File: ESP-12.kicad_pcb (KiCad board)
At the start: 2 copper layers, 30 x 34 mm, 16 parts, among them IC1 REG, P1 GPIO_1, P2 GPIO_2, P3 UART, P4 SPI, P5 P_IN, SW1 RESET, SW2 FLASH, U1 ESP-12E

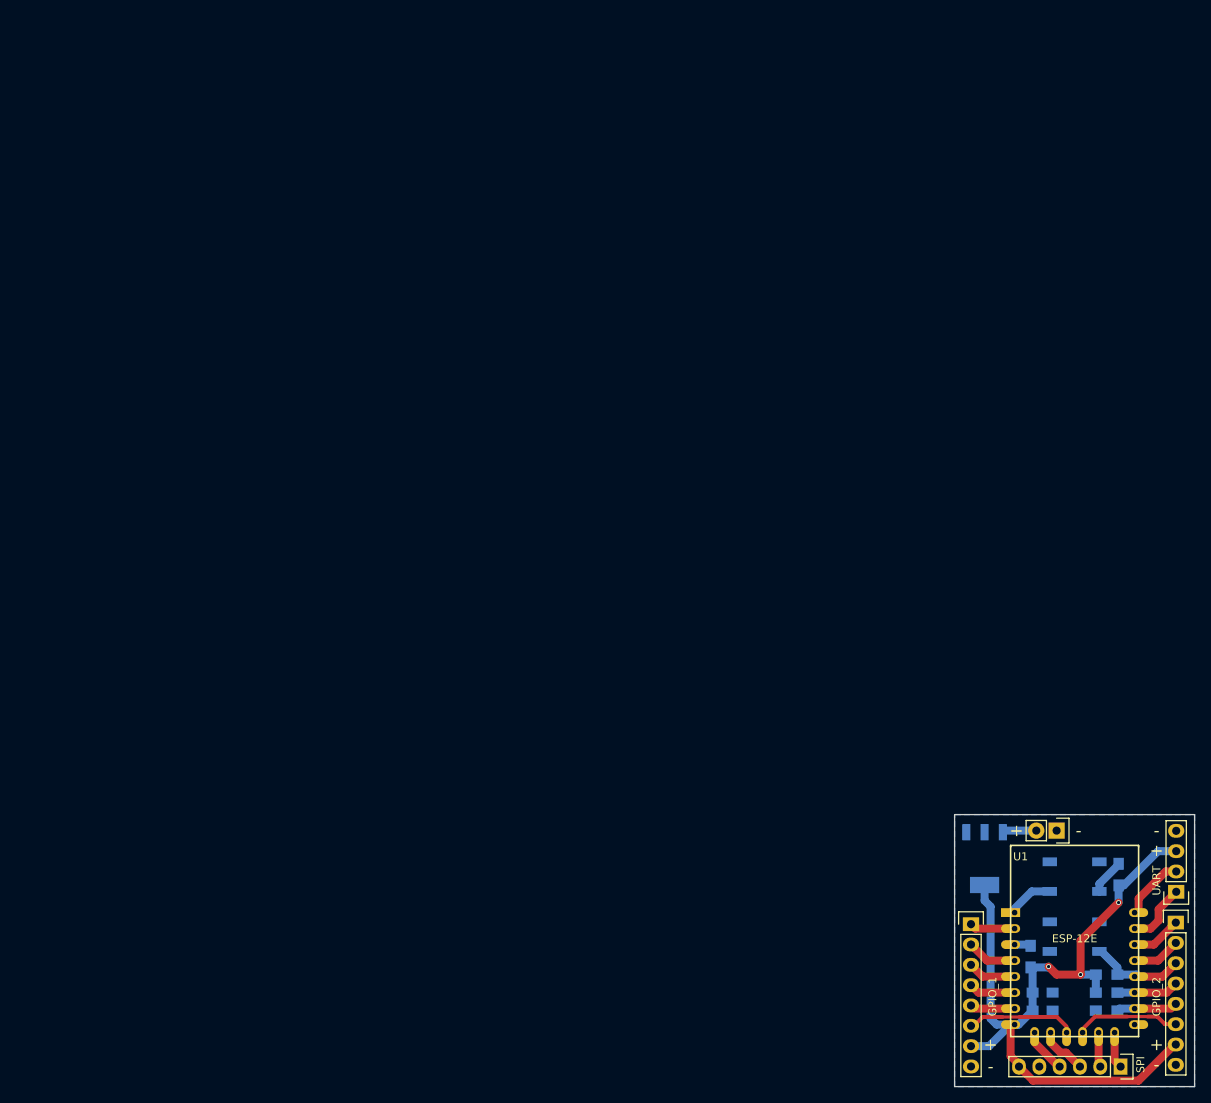
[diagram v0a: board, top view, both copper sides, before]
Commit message: Initial commit
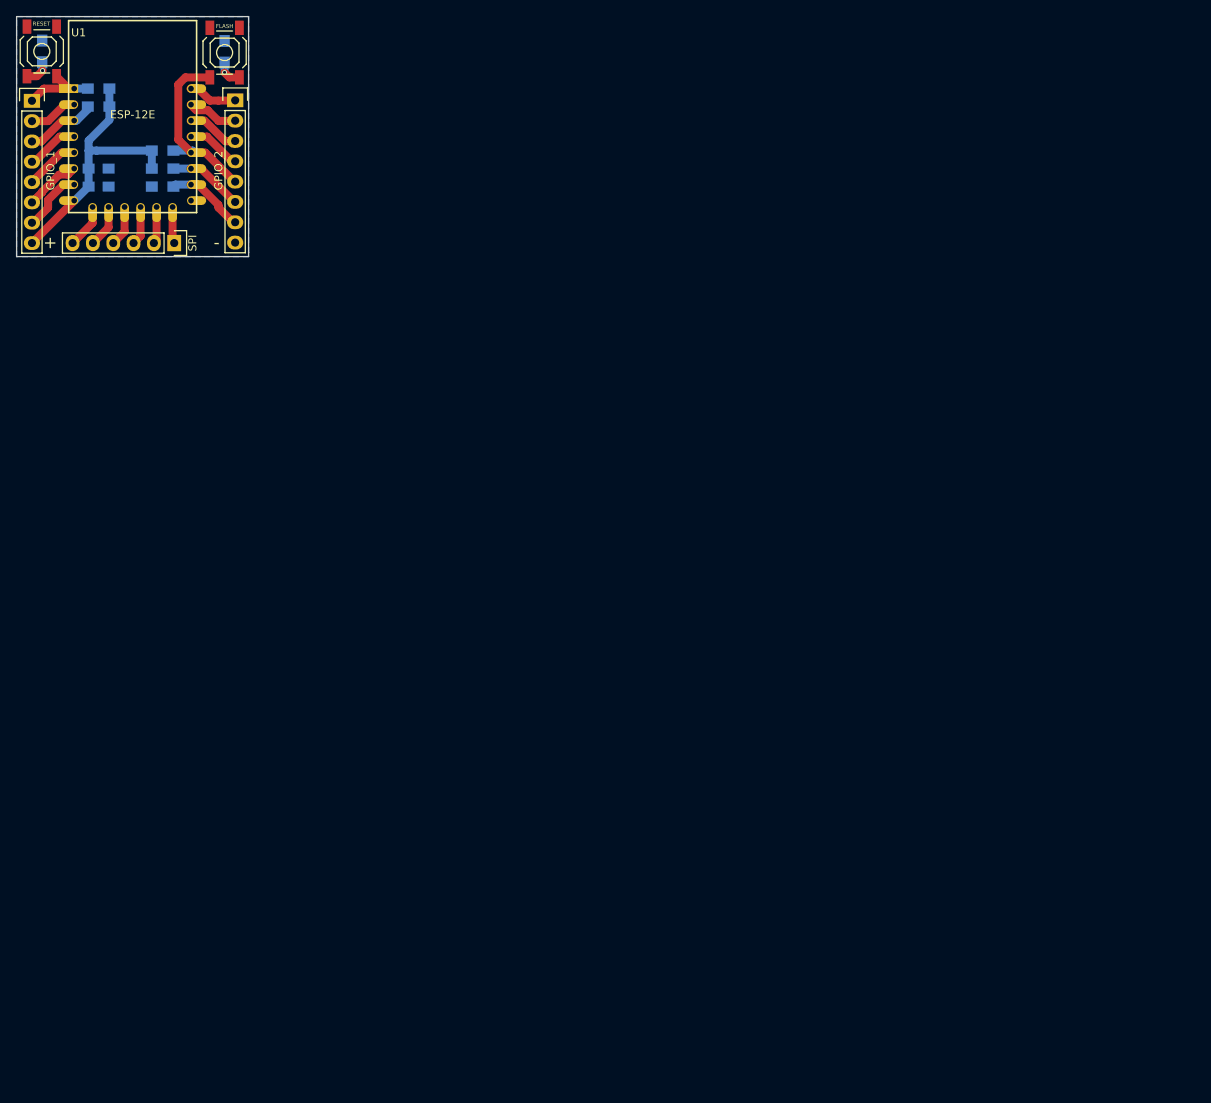
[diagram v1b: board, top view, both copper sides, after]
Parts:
- removed IC1: REG, TO_SOT_Packages_SMD:SOT-223
- removed P4: SPI, Pin_Headers:Pin_Header_Straight_1x06
- removed P5: P_IN, Pin_Headers:Pin_Header_Straight_1x02
- added R6: R, Resistors_SMD:R_0805_HandSoldering, B.Cu at (27.7, 24.1)
- added R7: R, Resistors_SMD:R_0805_HandSoldering, B.Cu at (50.5, 24.1)
- P3: value UART -> SPI; footprint Pin_Headers:Pin_Header_Straight_1x04 -> Pin_Headers:Pin_Header_Straight_1x06
- SW1, SW2: moved to F.Cu
- moved SW1 165.2 mm to (27.6, 24.1), turned to 270 degrees
- moved R1 161.0 mm to (34.8, 28.8), turned to 0 degrees
- moved R2 157.7 mm to (34.8, 31.0), turned to 0 degrees
- moved C2 156.6 mm to (34.8, 41.0)
- moved C3 156.6 mm to (34.8, 38.8)
- moved R3 156.6 mm to (42.8, 36.5)
- moved R4 156.6 mm to (42.8, 38.8)
- moved R5 156.6 mm to (42.8, 41.0)
- moved U1 156.4 mm to (31.0, 28.8)
- moved P2 156.2 mm to (51.8, 30.2)
- moved P1 156.1 mm to (26.4, 30.3)
- moved SW2 153.3 mm to (50.5, 24.2), turned to 90 degrees
- moved P3 149.2 mm to (44.2, 48.1), turned to 270 degrees
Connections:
- P1 pad 1: /ADC -> /RST
- P1 pad 2: /GPIO16 -> /ADC
- P1 pad 3: /GPIO14 -> /CH_PD
- P1 pad 4: /GPIO13 -> /GPIO16
- P1 pad 5: /GPIO12 -> /GPIO14
- P1 pad 6: /GPIO9 -> /GPIO12
- P1 pad 7: VCC -> /GPIO13
- P1 pad 8: GND -> VCC
- R1 pad 1: Net-(R1-Pad1) -> /RST
- R2 pad 1: Net-(R2-Pad1) -> /CH_PD
- SW1 pad 1: Net-(R1-Pad1) -> /RST
- SW1 pad 2: GND -> Net-(R6-Pad2)
- SW2 pad 2: GND -> Net-(R7-Pad2)
- U1 pad 1: Net-(R1-Pad1) -> /RST
- U1 pad 3: Net-(R2-Pad1) -> /CH_PD
- U1 pad 6: /GPIO13 -> /GPIO12
- U1 pad 7: /GPIO12 -> /GPIO13
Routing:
- net VCC: track 95.2 -> 34.4 mm, vias 3 -> 0
- net /GPIO0: track 12.1 -> 23.2 mm
- net Net-(R1-Pad1): track 10.5 -> 0.00 mm
- net /GPIO9: track 14.8 -> 4.89 mm
- net /RST: track 0.00 -> 9.59 mm
- net /GPIO10: track 13.9 -> 4.67 mm
- net /CH_PD: track 0.00 -> 9.24 mm
- net /GPIO15: track 6.81 -> 11.7 mm
- net /Vin: track 4.26 -> 0.00 mm
- net Net-(R7-Pad2): track 0.00 -> 3.35 mm, vias 0 -> 1
- net /GPIO2: track 7.77 -> 11.1 mm
- net Net-(R6-Pad2): track 0.00 -> 3.24 mm, vias 0 -> 1
- net Net-(R2-Pad1): track 3.06 -> 0.00 mm
- net /MISO: track 7.63 -> 5.12 mm
- net /GPIO13: track 5.34 -> 7.64 mm
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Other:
- board size 30 x 34 mm -> 29 x 30 mm
- board text added: "ESPBoardv1.0"
- board text added: "www.falseascension.xyz"
